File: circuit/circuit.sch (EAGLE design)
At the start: 16 parts, among them IC1 AT90S2313P, Q1 16MHz

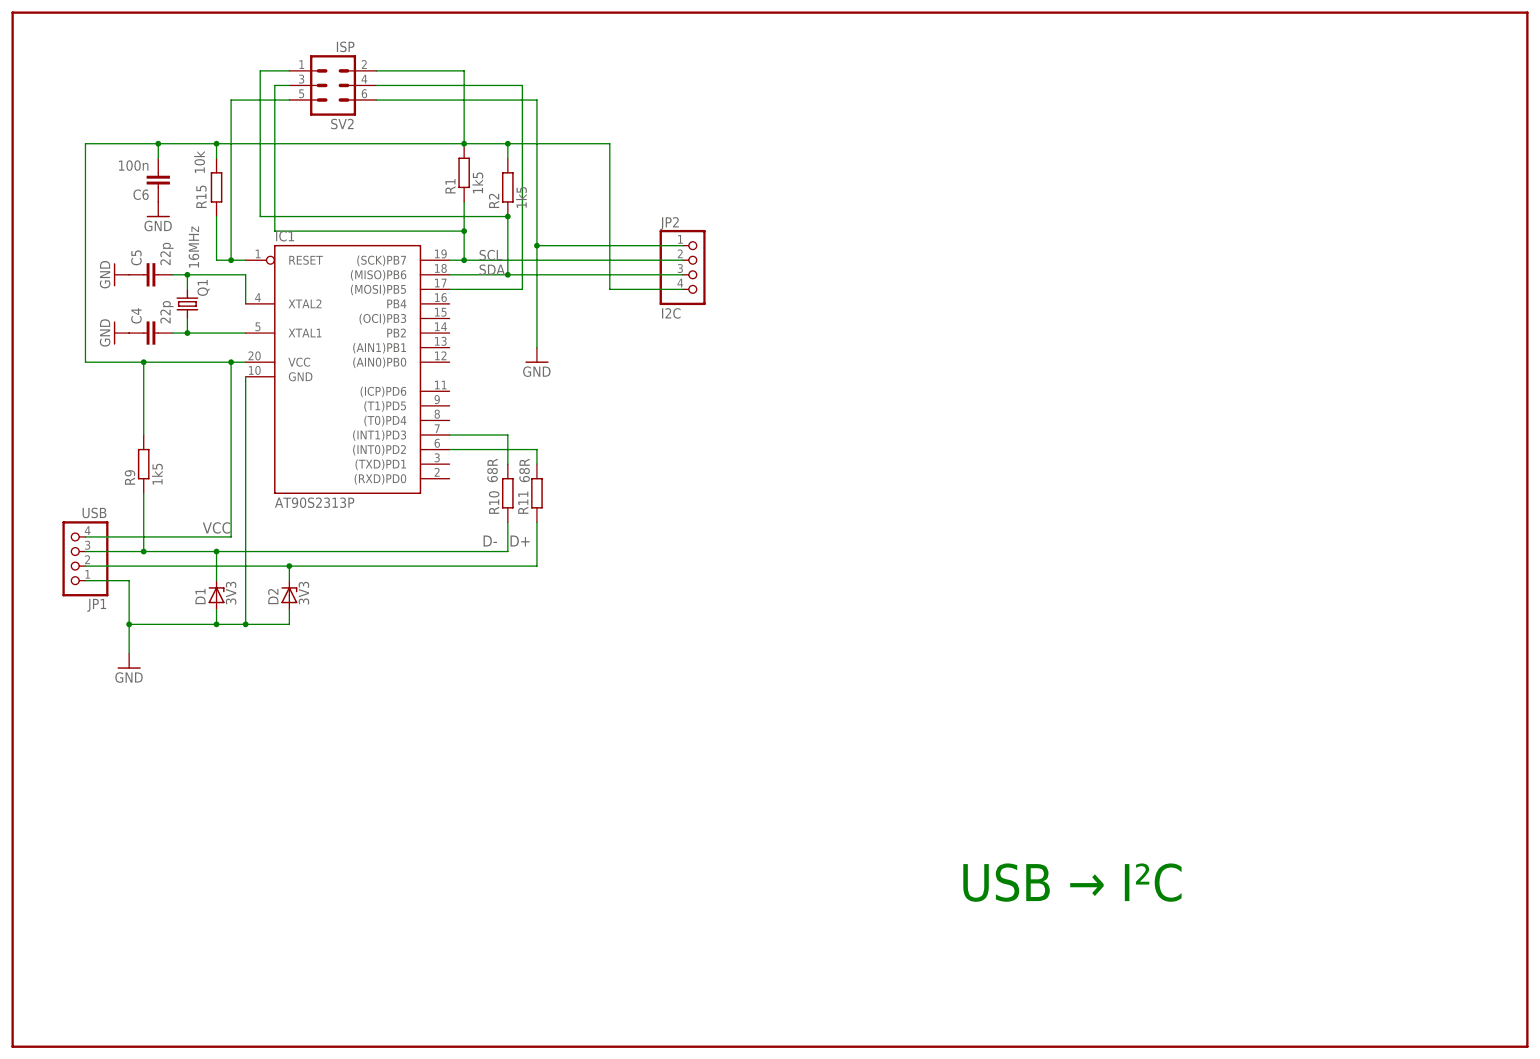
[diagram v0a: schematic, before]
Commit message: more layouting
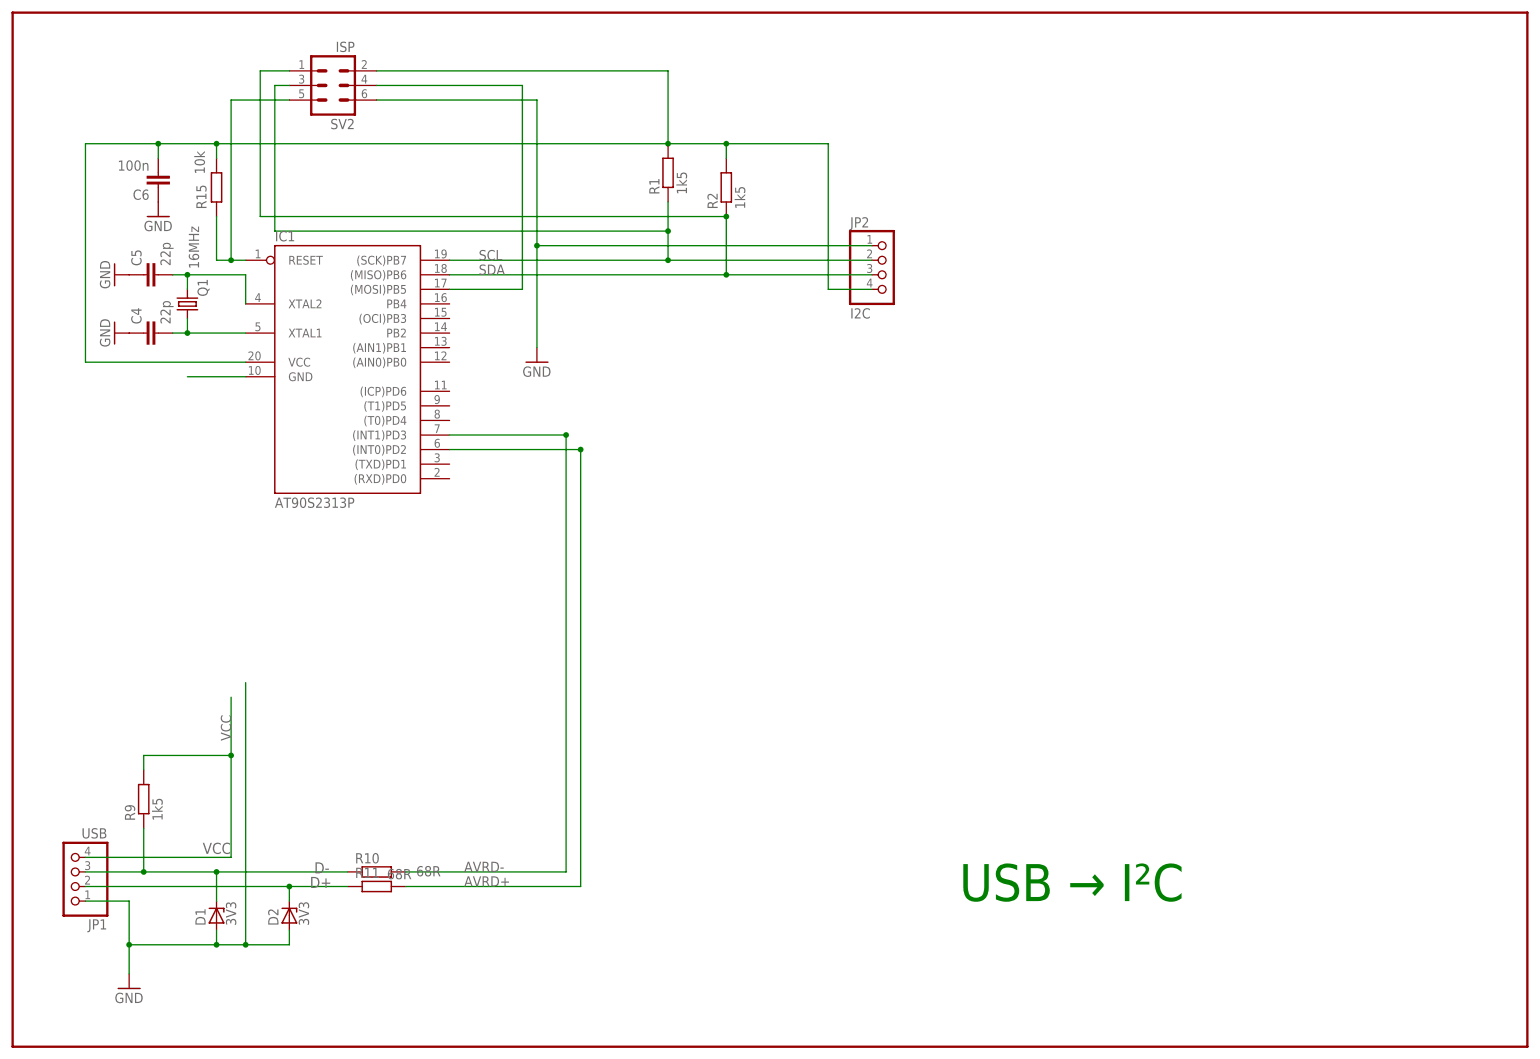
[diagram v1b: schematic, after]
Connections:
- net N$27 renamed AVRD+
- net N$41 renamed AVRD-
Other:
- moved on the sheet: D1, D2, JP1, JP2, R1, R10, R11, R2, R9
